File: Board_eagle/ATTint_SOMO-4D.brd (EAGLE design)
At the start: 32.1 x 31.1 mm, 18 parts, among them U1 SOMO-14D, U2 MAX1555, X2 STEREOJACK, X3 USB-SMD-NS

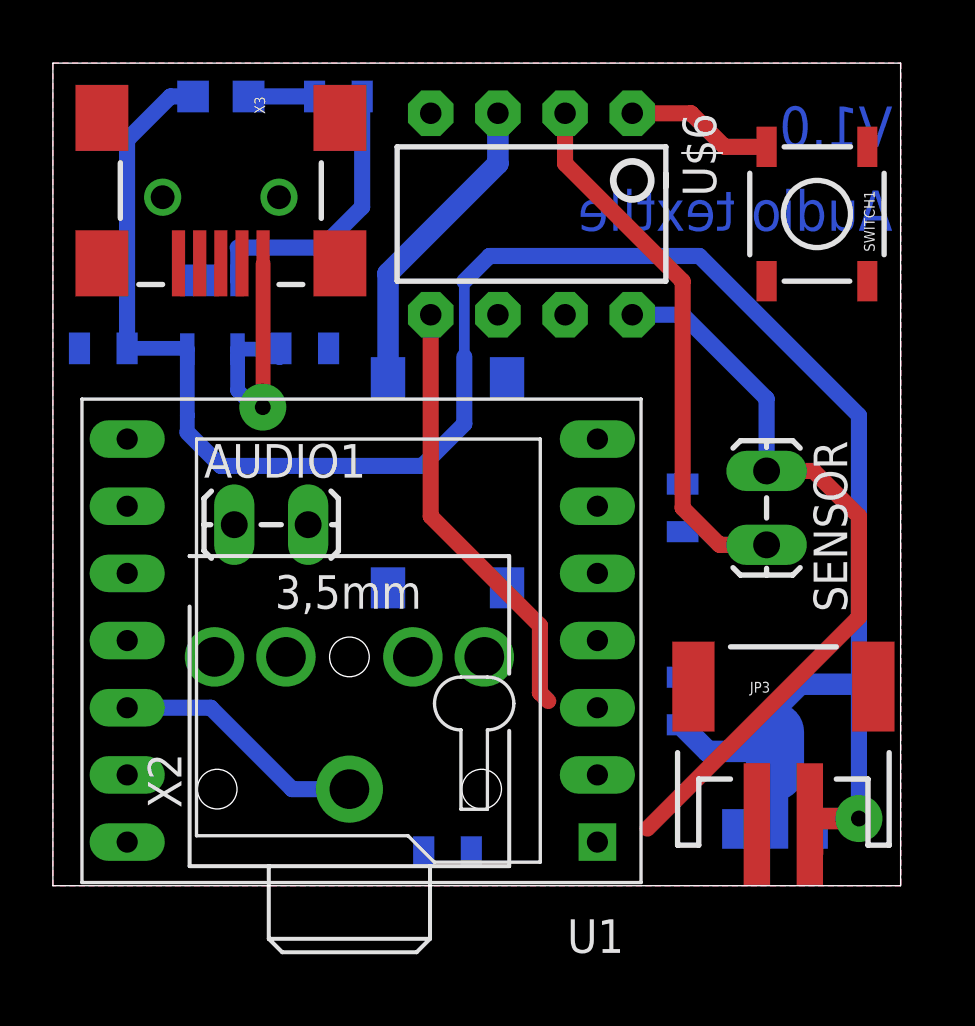
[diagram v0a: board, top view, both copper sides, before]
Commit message: Code cleaning
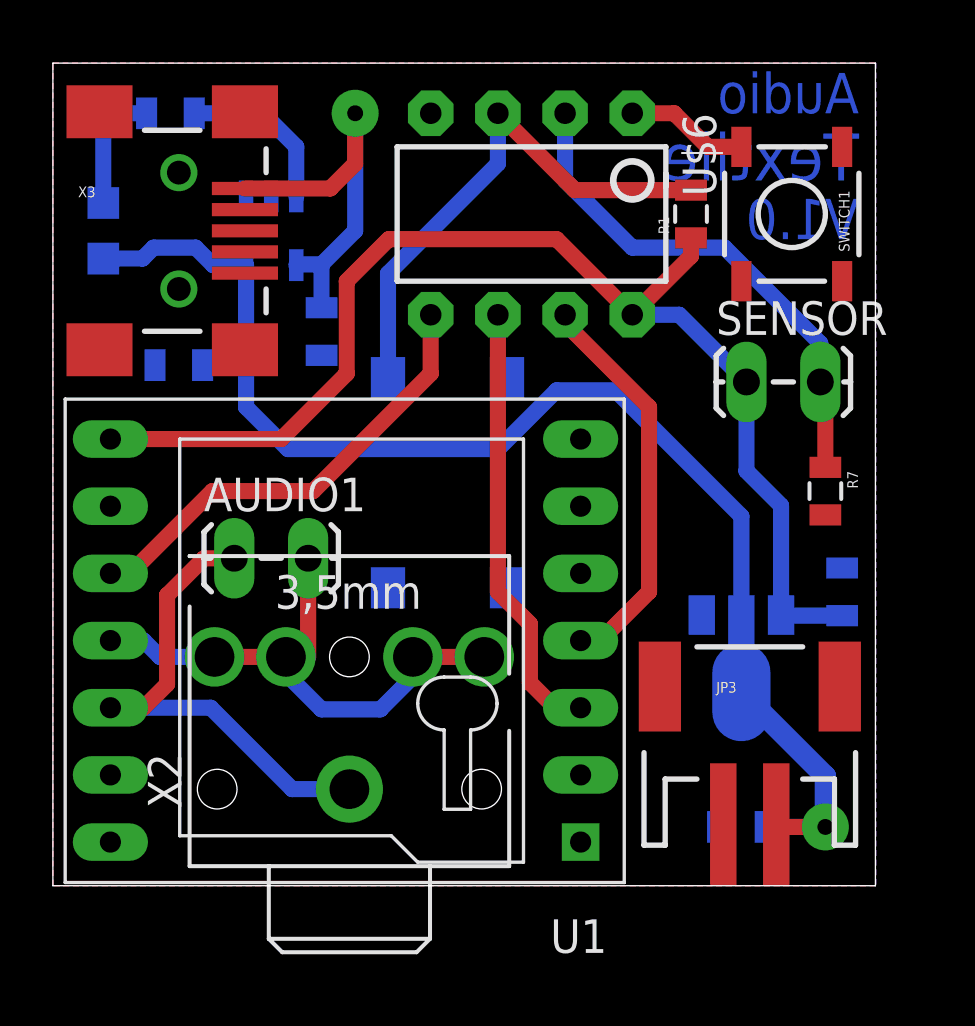
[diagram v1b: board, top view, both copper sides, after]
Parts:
- added R1: 1K, spark-fun:0805
- moved C1 17.9 mm to (29.8, 11.1), turned to 90 degrees
- moved LED1 6.75 mm to (1.91, 24.8), turned to 0 degrees
- moved R6 6.38 mm to (4.45, 29.2)
- moved R7 5.43 mm to (29.2, 14.9), flipped to the top
- moved C4 5.26 mm to (26.0, 2.22), turned to 0 degrees
- moved U$3 4.32 mm to (26.0, 8.26), turned to 180 degrees
- moved U2 3.88 mm to (8.26, 24.8)
- moved SENSOR 3.55 mm to (26.4, 19.1), turned to 0 degrees
- moved C9 2.93 mm to (4.76, 19.7)
- moved X3 2.03 mm to (4.76, 24.8), turned to 0 degrees
- moved AUDIO1 1.27 mm to (6.99, 12.4)
- moved JP3 1.27 mm to (26.4, 6.03)
- moved SWITCH1 0.95 mm to (27.9, 25.4)
- moved C7 0.90 mm to (10.2, 21.0), turned to 270 degrees
- moved U1 0.63 mm to (10.8, 8.89)
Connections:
- net CLOCK: now also U$6.6; no longer U$6.5
- net DATA: now also U$6.7; no longer U$6.6
- net RESET: now also U$6.5; no longer U$6.7
- net SWITCH: now also R1.2
- net VCC: now also R1.1
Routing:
- net VCHARGE: track 85.1 -> 52.4 mm
- net AUDIO_B: track 0.00 -> 21.4 mm
- net VCC: track 28.5 -> 47.0 mm
- net RESET: track 0.00 -> 17.5 mm
- net DATA: track 0.00 -> 15.1 mm
- net AUDIO_A: track 9.68 -> 19.3 mm
- net SWITCH: track 11.7 -> 20.2 mm
- net N$6: track 10.4 -> 15.3 mm
- net N$7: track 10.8 -> 6.26 mm
- net N$8: track 2.49 -> 4.66 mm
- net SENSOR: track 20.5 -> 19.5 mm
- net NRESET: track 5.61 -> 4.65 mm
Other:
- board size 32.1 x 31.1 mm -> 31.1 x 31.1 mm
- board text added: "Audio"
- board text added: "Textile"
- board text removed: "Audio textile"
